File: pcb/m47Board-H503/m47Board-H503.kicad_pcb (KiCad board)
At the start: 2 copper layers, 44 parts, among them J1 USB_C_Receptacle_USB2.0_14P, J2 Conn_01x05_Pin, J3 Conn_01x10_Pin, J4 Conn_01x10_Pin, J5 Conn_01x09_Pin, J6 Conn_01x06_Pin, SW1 SW_Push, SW2 SW_Push, SW3 SW_Push, U1 AP2114H-3.3TRG1, U2 STM32H503CBTx, U3 USBLC6-2SC6, Y1 CX3225FB16000F0FZZH1 16MHz, Y2 ABS07-32.768KHZ-T

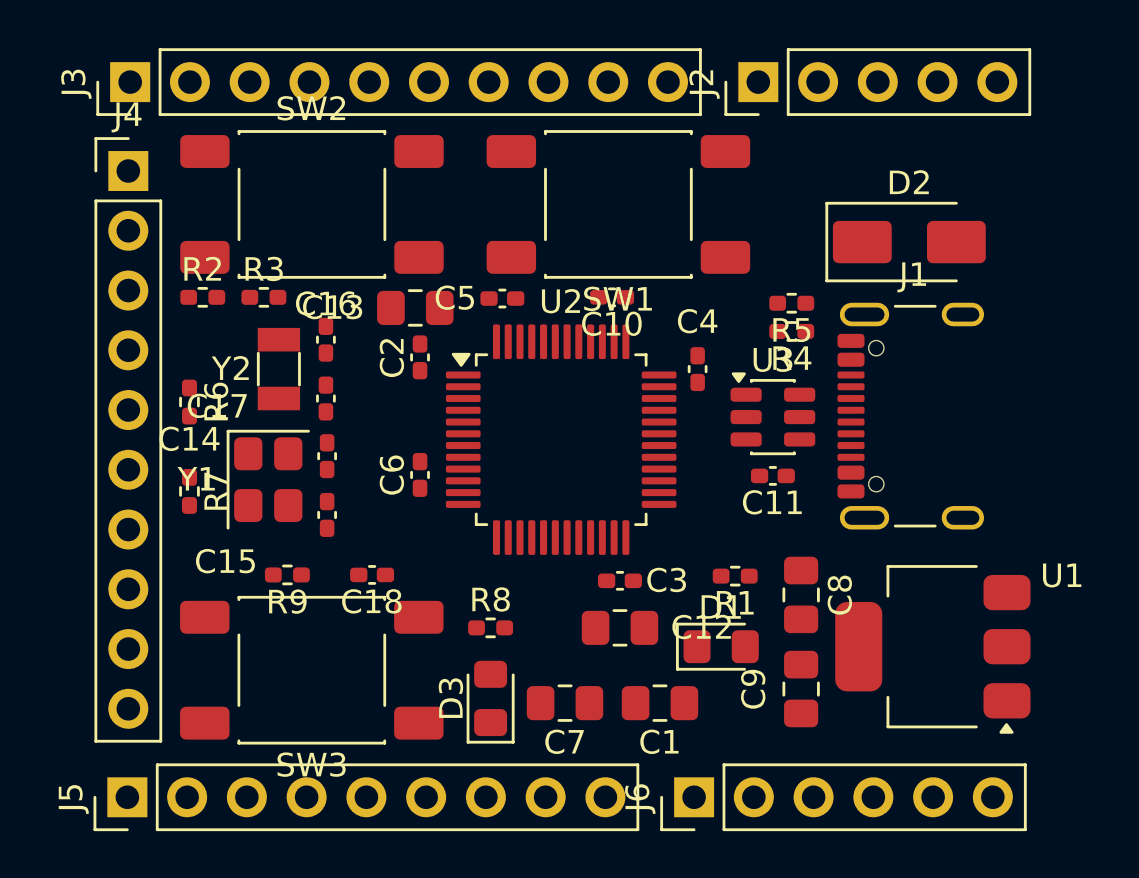
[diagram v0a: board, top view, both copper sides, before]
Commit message: m47Board-H503 PCB layout update
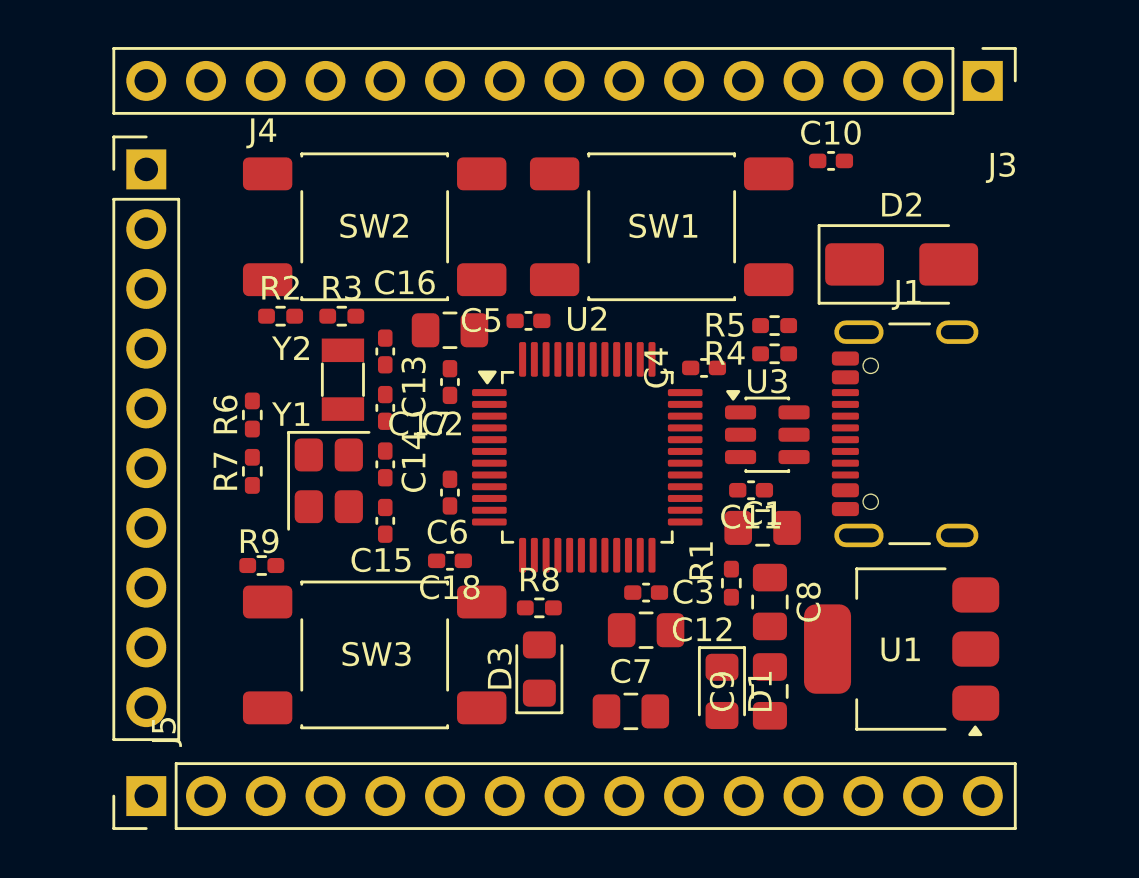
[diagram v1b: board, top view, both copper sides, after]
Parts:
- removed J2: Conn_01x05_Pin, Connector_PinHeader_2.54mm:PinHeader_1x05_P2.54mm_Vertical
- removed J6: Conn_01x06_Pin, Connector_PinHeader_2.54mm:PinHeader_1x06_P2.54mm_Vertical
- J3: value Conn_01x10_Pin -> Conn_01x15_Pin; footprint Connector_PinHeader_2.54mm:PinHeader_1x10_P2.54mm_Vertical -> Connector_PinHeader_2.54mm:PinHeader_1x15_P2.54mm_Vertical
- J5: value Conn_01x09_Pin -> Conn_01x15_Pin; footprint Connector_PinHeader_2.54mm:PinHeader_1x09_P2.54mm_Vertical -> Connector_PinHeader_2.54mm:PinHeader_1x15_P2.54mm_Vertical
- moved J3 36.2 mm to (166.0, 83.6), turned to -90 degrees
- moved C10 11.0 mm to (159.5, 87.0), turned to 0 degrees
- moved C1 8.63 mm to (156.6, 102.6), turned to 0 degrees
- moved R2 3.41 mm to (136.1, 93.6)
- moved R3 3.41 mm to (138.7, 93.6)
- moved C18 3.36 mm to (143.3, 104.0)
- moved SW2 2.83 mm to (140.1, 89.8)
- moved C7 2.82 mm to (151.0, 110.4), turned to 0 degrees
- moved R7 2.81 mm to (134.9, 100.2)
- moved Y2 2.76 mm to (138.8, 96.3)
- moved SW3 2.75 mm to (140.1, 108.0)
- moved R6 2.73 mm to (134.9, 97.8)
- moved Y1 2.57 mm to (138.2, 100.6)
- moved C16 2.57 mm to (140.6, 95.1), turned to 90 degrees
- moved C17 2.55 mm to (140.6, 97.5)
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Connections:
- J3 pad 1: unconnected-(J3-Pin_1-Pad1) -> +3.3V
- J3 pad 2: unconnected-(J3-Pin_2-Pad2) -> /SWCLK
- J3 pad 3: unconnected-(J3-Pin_3-Pad3) -> GND
- J3 pad 4: unconnected-(J3-Pin_4-Pad4) -> /SWDIO
- J3 pad 5: unconnected-(J3-Pin_5-Pad5) -> /NRST
